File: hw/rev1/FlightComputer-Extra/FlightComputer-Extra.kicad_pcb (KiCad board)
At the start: 2 copper layers, 128 x 16.9 mm, 22 parts, among them J1 SJ-43617-SMT, J2 Conn_01x10, J3 Conn_01x10, J4 IPEX_IPX, J5 Conn_DEBUG, U1 Teseo-LIV3F

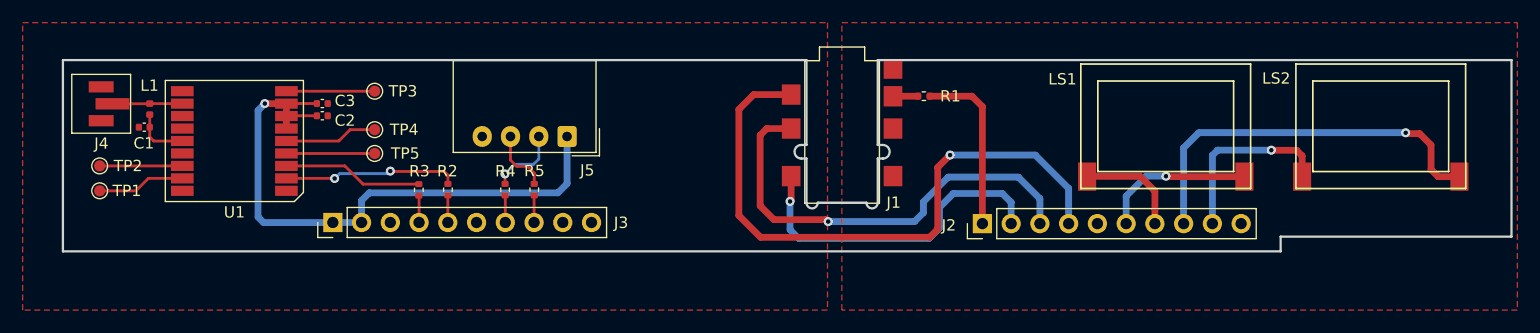
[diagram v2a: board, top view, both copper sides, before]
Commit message: ...
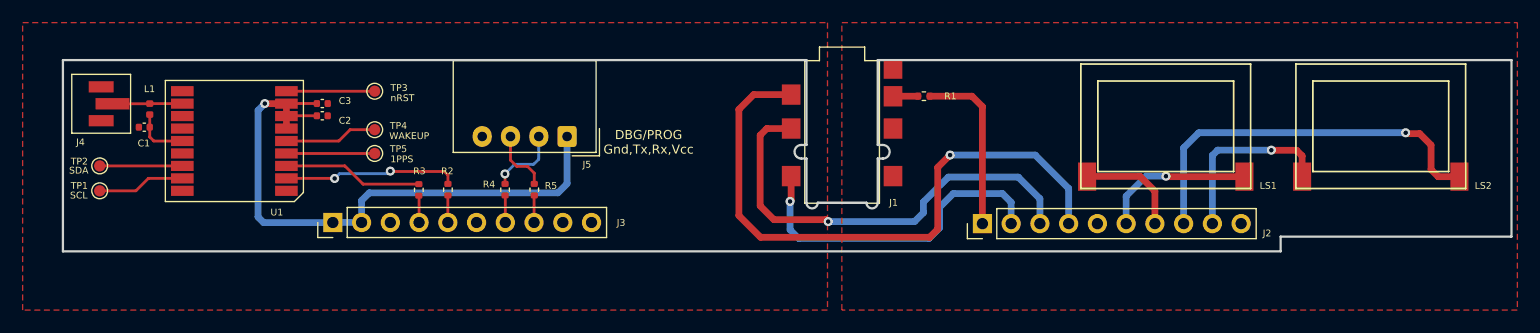
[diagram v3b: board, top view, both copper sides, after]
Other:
- board text added: "1PPS"
- board text added: "DBG/PROG Gnd,Tx,Rx,Vcc"
- board text added: "SCL"
- board text added: "SDA"
- board text added: "WAKEUP"
- board text added: "nRST"
